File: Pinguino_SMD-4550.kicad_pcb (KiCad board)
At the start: 2 copper layers, 50 x 25 mm, 51 parts, among them P1 uUSB, P10 CONN_01X01, P11 CONN_01X01, P12 CONN_01X01, P13 CONN_01X01, P14 CONN_01X01, P15 CONN_01X01, P16 CONN_01X01, P17 CONN_01X01, P18 CONN_01X01, P19 CONN_01X01, P2 CONN_01X01, P20 CONN_01X01, P21 CONN_01X01, P22 CONN_01X01, P23 CONN_01X01, P24 CONN_01X01, P25 CONN_01X01, P26 CONN_01X01, P27 CONN_01X01, P28 CONN_01X01, P29 CONN_01X01, P3 CONN_01X01, P30 CONN_01X01, P31 CONN_01X01, P32 CONN_01X01, P33 CONN_01X01, P34 CONN_01X01, P35 CONN_01X01, P36 CONN_01X01, P37 CONN_01X01, P38 CONN_01X01, P4 CONN_01X01, P5 CONN_01X01, P6 CONN_01X01, P7 CONN_01X01, P8 CONN_01X01, P9 CONN_01X01, SW1 Reset, U1 PIC18(L)F4550-I/PT, Y1 Crystal

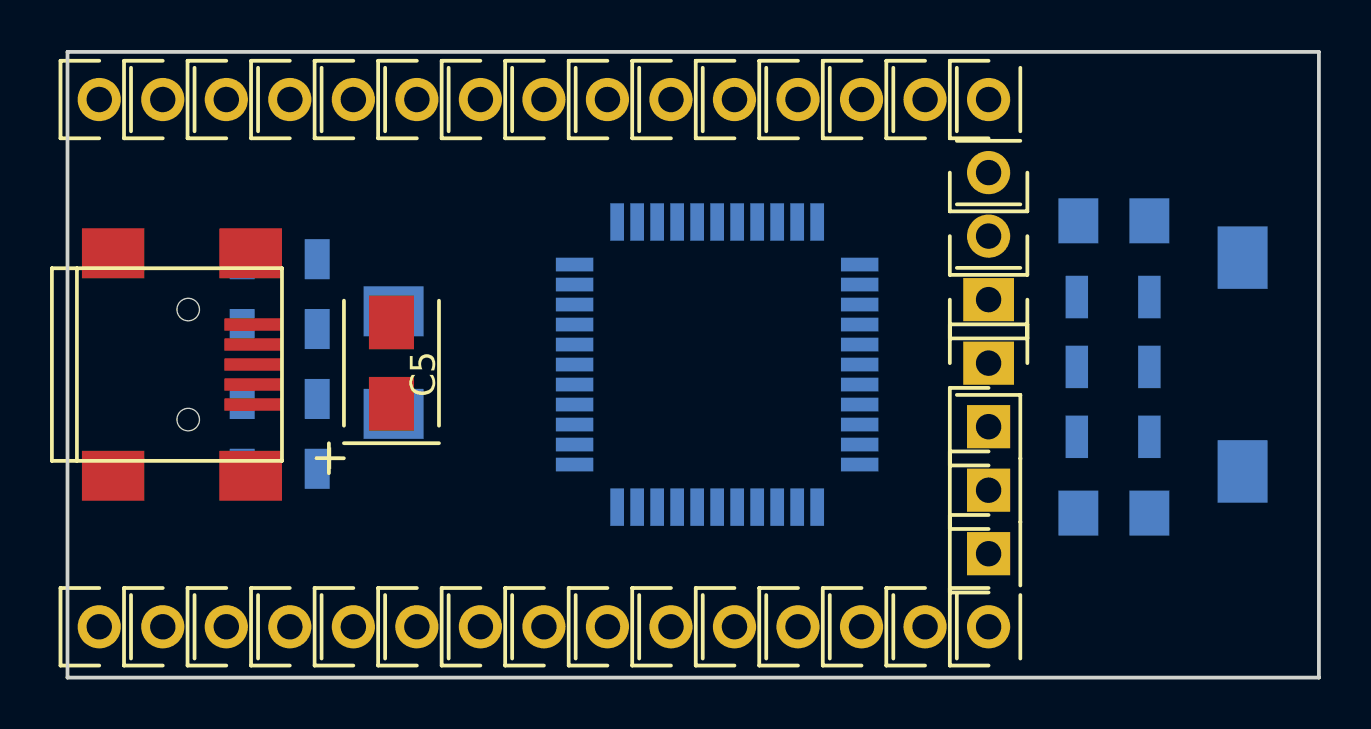
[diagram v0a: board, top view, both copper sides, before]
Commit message: Autoruting
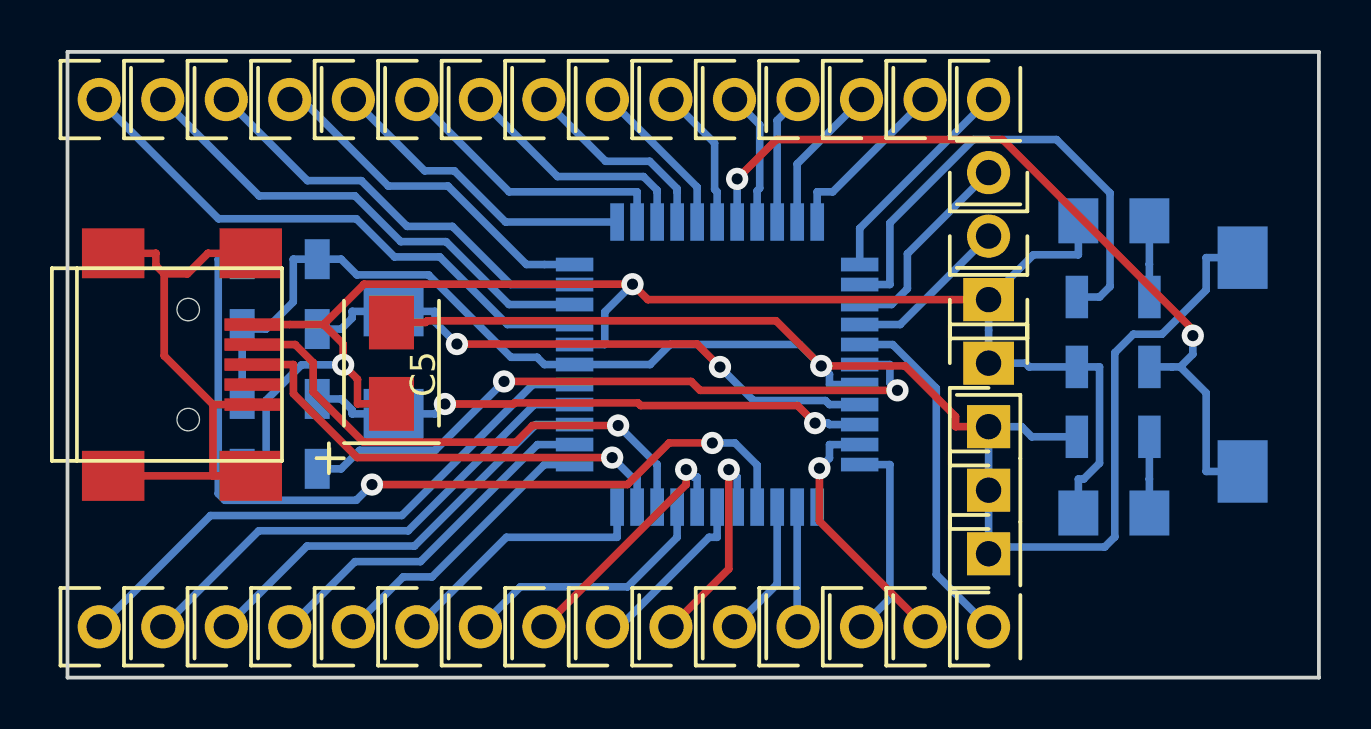
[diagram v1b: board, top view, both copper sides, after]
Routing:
- net GND: track 0.00 -> 87.3 mm, vias 0 -> 1
- net VCC: track 0.00 -> 65.9 mm, vias 0 -> 2
- net /VUSB: track 0.00 -> 35.0 mm, vias 0 -> 2
- net /MCLR: track 0.00 -> 32.7 mm, vias 0 -> 2
- net Net-(C3-Pad2): track 0.00 -> 27.2 mm, vias 0 -> 2
- net /OSC1: track 0.00 -> 23.9 mm, vias 0 -> 2
- net /PIN28: track 0.00 -> 23.0 mm
- net /PIN0/SDA: track 0.00 -> 22.7 mm
- net /OSC0: track 0.00 -> 22.6 mm, vias 0 -> 2
- net Net-(P1-Pad5): track 0.00 -> 22.5 mm
- net /D-: track 0.00 -> 21.1 mm, vias 0 -> 1
- net /PIN27: track 0.00 -> 20.1 mm
- net /RA4: track 0.00 -> 20.0 mm
- net /PIN1/SCL: track 0.00 -> 19.9 mm
- net /D+: track 0.00 -> 19.1 mm, vias 0 -> 1
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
